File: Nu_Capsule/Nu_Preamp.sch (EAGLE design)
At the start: 15 parts, among them U1 OPA209AIDVBR

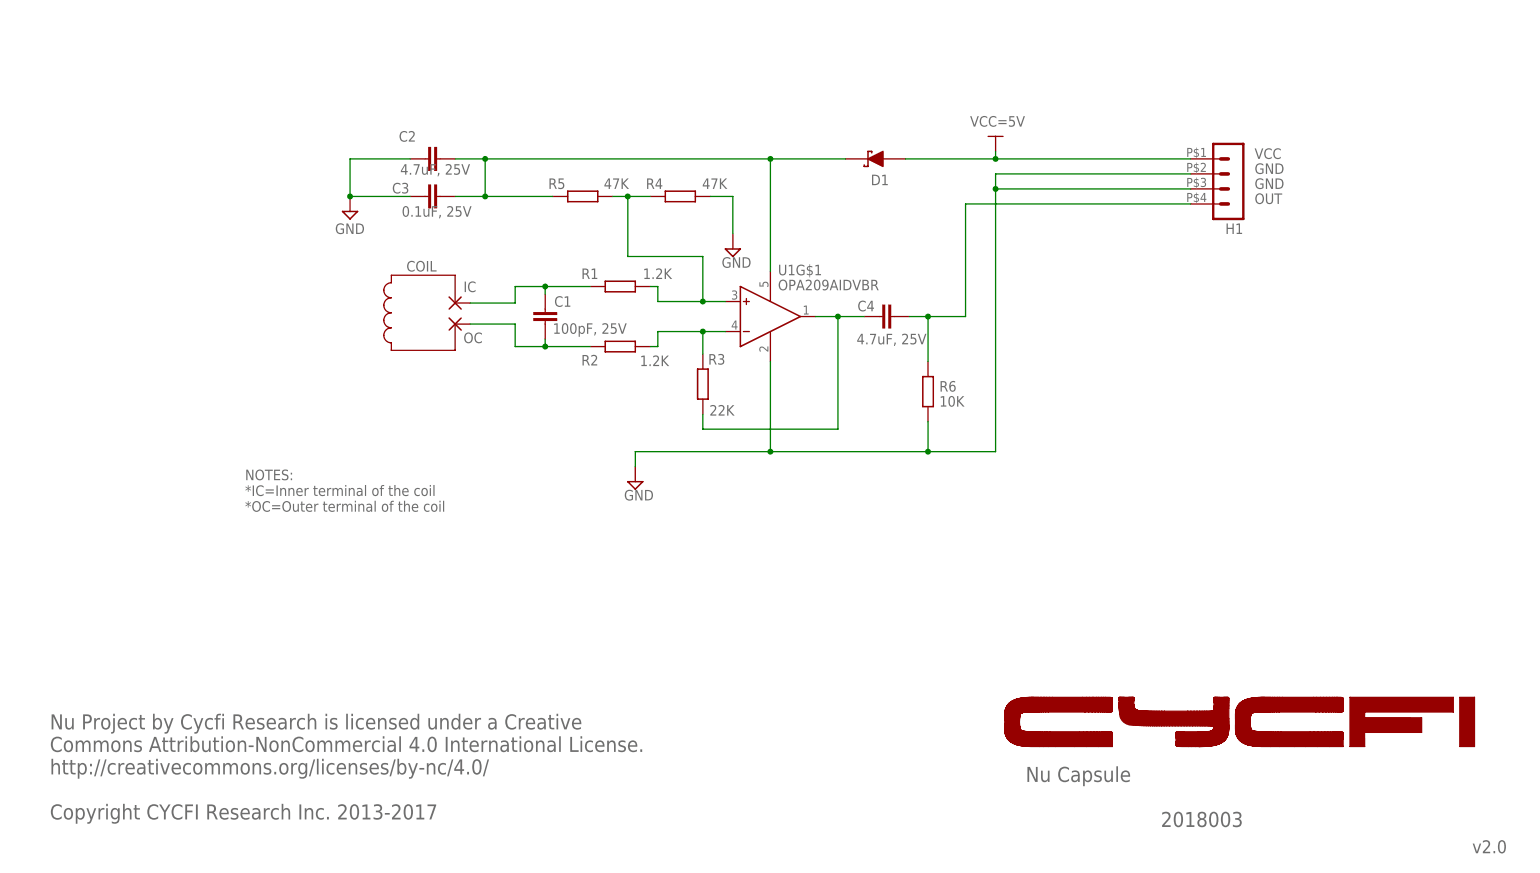
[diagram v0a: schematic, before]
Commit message: Updated Nu Preamp Files
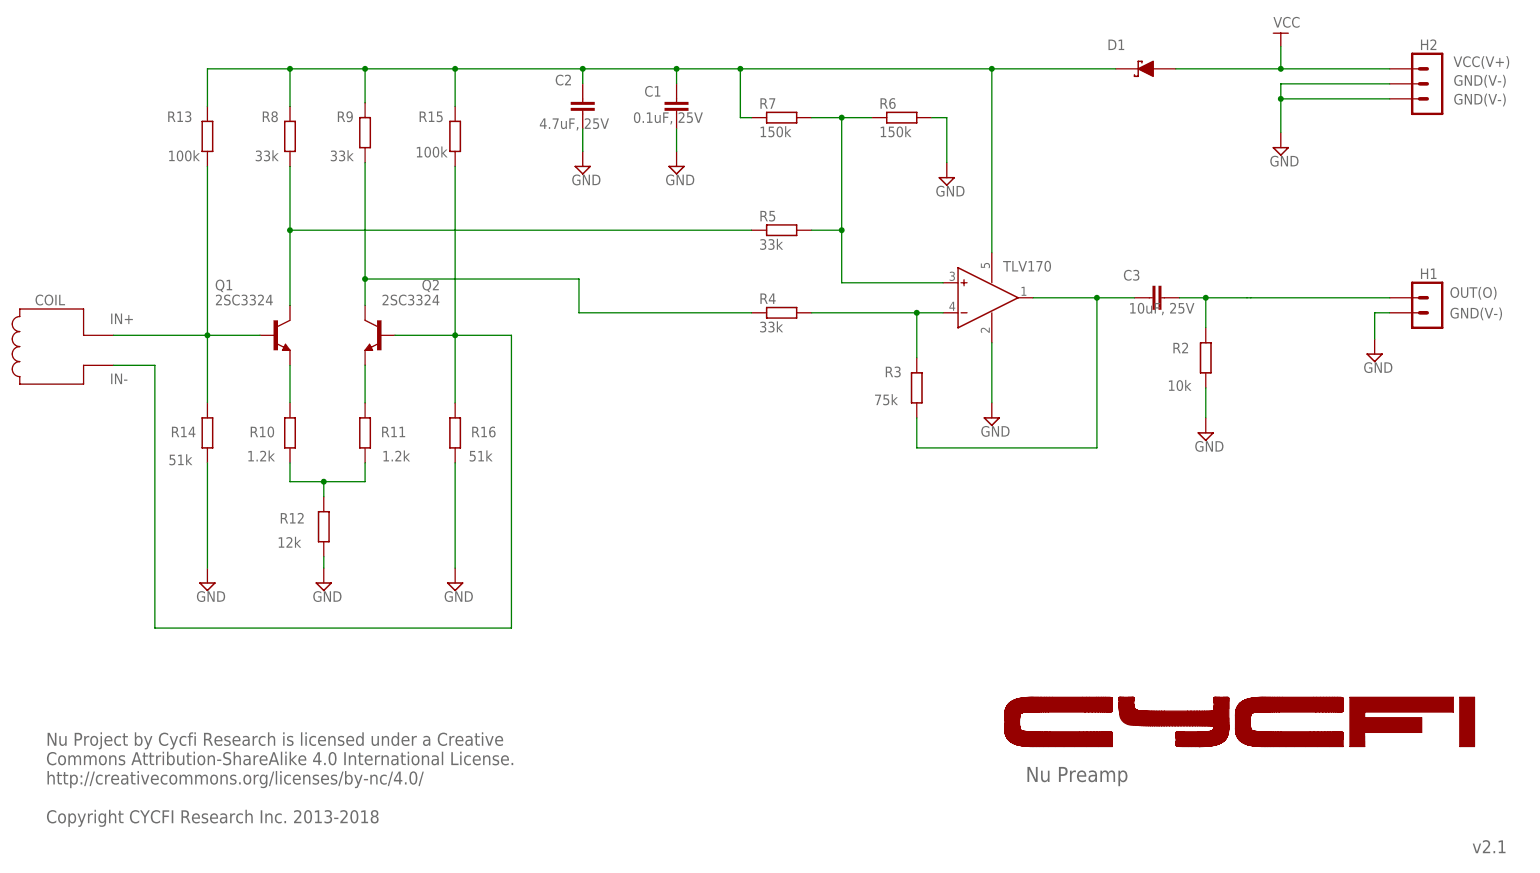
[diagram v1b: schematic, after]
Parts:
- removed C4: 4.7uF, 25V, rcl:C-EUC0603
- removed IC, OC: (no value), wirepad:1,6/0,8
- removed R1: 1.2K, resistor:R-EU_R0402
- added H2: 3P-2MM-TH-MALE, CYCFI_Con:3P-2MM-TH-MALE
- added Q1, Q2: 2SC3324, CYCFI_semicon:2SC3324
- added R10, R11: 1.2k, rcl:R-EU_R0402
- added R12: 12k, rcl:R-EU_R0402
- added R13, R15: 100k, rcl:R-EU_R0402
- added R14, R16: 51k, rcl:R-EU_R0402
- added R7: 150k, resistor:R-EU_R0402
- added R8, R9: 33k, rcl:R-EU_R0402
- C1: value 100pF, 25V -> 0.1uF, 25V
- C3: value 0.1uF, 25V -> 10uF, 25V; device rcl:C-EUC0402 -> rcl:C0603_NK
- H1: value 4P_ZIF_59453-041110EDHLF -> 2P-2MM-TH-MALE; device CYCFI_Con:4P_ZIF_59453-041110EDHLF -> CYCFI_Con:2P-2MM-TH-MALE
- R2: value 1.2K -> 10k; device resistor:R-EU_R0402 -> rcl:R-EU_R0402
- R3: value 22K -> 75k
- R4, R5: value 47K -> 33k
- R6: value 10K -> 150k
- U1: value OPA209AIDVBR -> TLV170; device CYCFI_semicon:OPA209DBVR -> CYCFI_semicon:TLV170
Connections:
- removed net N$2: C1.1, IC.P, R1.1
- removed net N$4: C1.2, OC.P, R2.1
- removed net N$7: R2.2, R3.1, U1G$1.IN-
- removed net OUT: C4.2, H1.4, R6.2
- removed net VCC: C2.2, C3.2, D1.C, R5.1, U1G$2.V+
- new net IN+: Q1.B, R13.1, R14.2
- new net IN-: Q2.B, R15.1, R16.2
- new net N$10: Q2.E, R11.2
- new net N$13: R10.1, R11.1, R12.2
- new net N$14: R5.2, R6.1, R7.2, U1G$1.IN+
- new net N$15: R3.2, R4.2, U1G$1.IN-
- new net N$16: C3.1, R3.1, U1G$1.OUT
- new net N$19: D1.A, H2.1
- new net N$9: Q1.E, R10.2
- new net VCC1: C1.1, C2.2, D1.C, R13.2, R15.2, R7.1, R8.2, R9.2, U1G$2.V+
- net GND: now also C1.2, H2.2, H2.3, R12.1, R14.1, R16.1, R2.1, R6.2; no longer C3.1, H1.3, R4.2, R6.1
- net N$1: now also C3.2, R2.2; no longer D1.A
- net N$5: now also Q1.C, R5.1, R8.1; no longer C4.1, R3.2, U1G$1.OUT
- net N$6: now also Q2.C, R9.1; no longer R1.2, R5.2, U1G$1.IN+
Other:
- note added: "GND(V-)"
- note added: "IN+"
- note added: "IN-"
- note added: "Nu Preamp"
- note added: "Nu Project by Cycfi Research is licensed under a Creative Commons Attribution-ShareAlike 4.0 International License. http://creativecommons.org/licenses/by-nc/4.0/ Copyright CYCFI Research Inc. 2013-2018"
- note added: "OUT(O)"
- note added: "VCC(V+)"
- note added: "v2.1"
- note removed: "2018003"
- note removed: "GND"
- note removed: "NOTES: *IC=Inner terminal of the coil *OC=Outer terminal of the coil"
- note removed: "Nu Capsule"
- note removed: "Nu Project by Cycfi Research is licensed under a Creative Commons Attribution-NonCommercial 4.0 International License. http://creativecommons.org/licenses/by-nc/4.0/ Copyright CYCFI Research Inc. 2013-2017"
- note removed: "OUT"
- note removed: "VCC=5V"
- note removed: "v2.0"
- moved on the sheet: C1, C2, C3, D1, R2, R3, R4, R5, R6
